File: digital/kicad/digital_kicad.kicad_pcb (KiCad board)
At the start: 2 copper layers, 14 parts, among them Q1 2N3904, Q2 2N3904, Q4 2N3904, SW1 SW_SPST

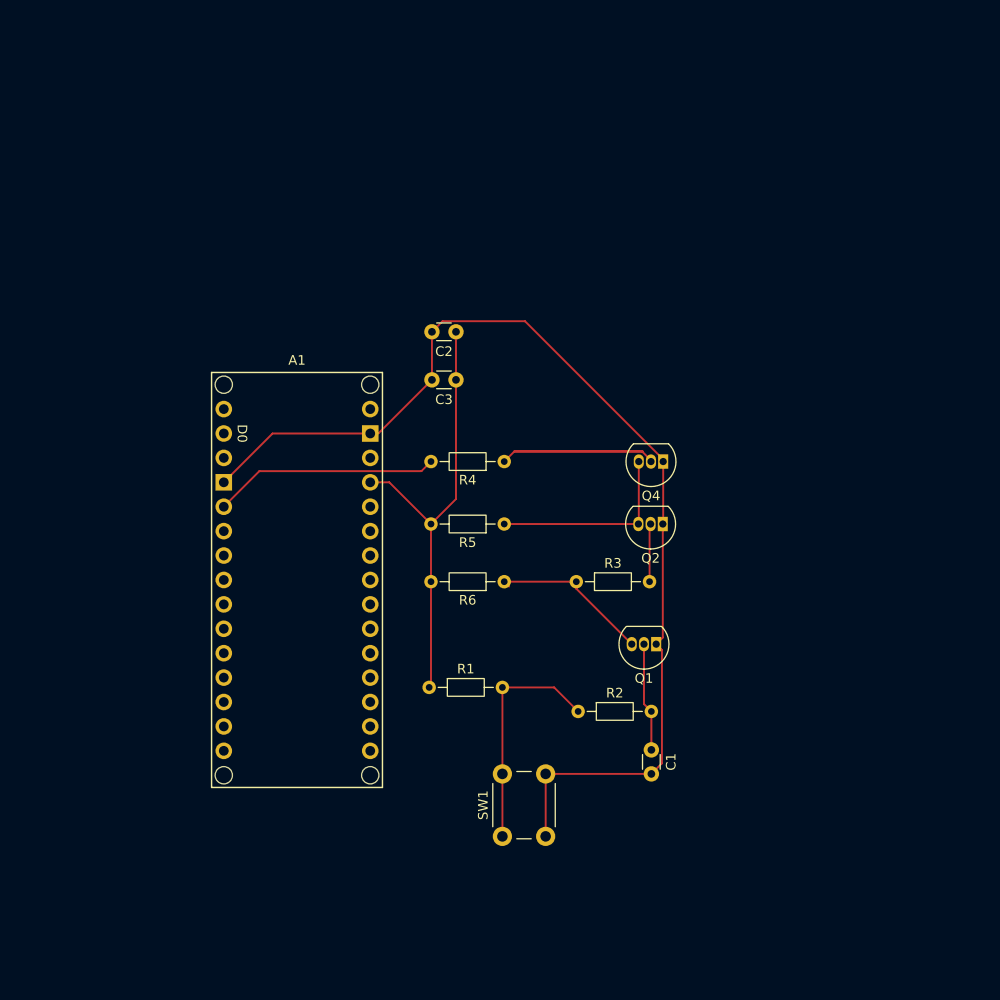
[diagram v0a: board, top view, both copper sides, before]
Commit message: kicad + pcb scheme review
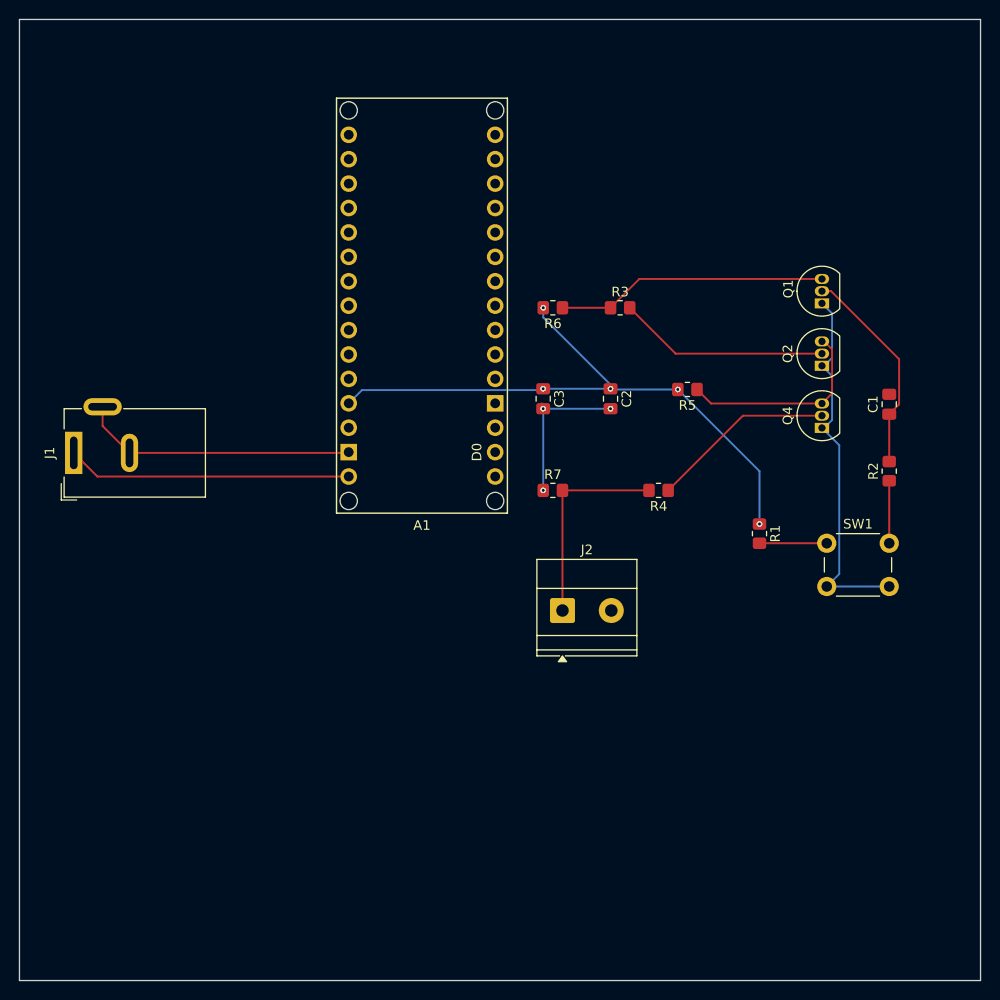
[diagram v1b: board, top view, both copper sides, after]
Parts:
- added J1: Barrel_Jack_Switch, Connector_BarrelJack:BarrelJack_Wuerth_6941xx301002, F.Cu at (105.7, 74.1)
- added J2: Screw_Terminal_01x02, TerminalBlock_Phoenix:TerminalBlock_Phoenix_MKDS-1,5-2-5.08_1x02_P5.08mm_Horizontal, F.Cu at (156.5, 90.5)
- added R7: 33k, Resistor_SMD:R_0805_2012Metric_Pad1.20x1.40mm_HandSolder, F.Cu at (155.5, 78.0)
- C1, C2, C3: footprint Capacitor_THT:C_Disc_D3.0mm_W1.6mm_P2.50mm -> Capacitor_SMD:C_0805_2012Metric_Pad1.18x1.45mm_HandSolder
- R1, R2, R3, R4, R5, R6: footprint Resistor_THT:R_Axial_DIN0204_L3.6mm_D1.6mm_P7.62mm_Horizontal -> Resistor_SMD:R_0805_2012Metric_Pad1.20x1.40mm_HandSolder
- moved A1 72.9 mm to (141.9, 37.2), turned to 180 degrees
- moved SW1 45.5 mm to (184.0, 83.5), turned to 0 degrees
- moved C1 43.7 mm to (190.5, 69.0), turned to 90 degrees
- moved R2 40.9 mm to (190.5, 76.0), turned to 90 degrees
- moved Q1 39.4 mm to (183.5, 58.5), turned to 90 degrees
- moved R1 37.9 mm to (177.0, 82.5), turned to -90 degrees
- moved R6 28.9 mm to (155.5, 59.0)
- moved R3 28.9 mm to (162.5, 59.0)
- moved R5 23.6 mm to (169.5, 67.5)
- moved Q2 23.3 mm to (183.5, 65.0), turned to 90 degrees
- moved C2 17.5 mm to (161.5, 68.5), turned to -90 degrees
- moved Q4 16.9 mm to (183.5, 71.5), turned to 90 degrees
- moved R4 16.3 mm to (166.5, 78.0)
- moved C3 9.28 mm to (154.5, 68.5), turned to -90 degrees
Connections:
- A1 pad D2: Net-(A1-D2_INT0) -> unconnected-(A1-D2_INT0-PadD2)
- A1 pad VIN: unconnected-(A1-PadVIN) -> /VDC
- R4 pad 2: Net-(A1-D2_INT0) -> Net-(J2-Pin_1)
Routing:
- net /VDC: track 0.00 -> 29.6 mm
- net GND: track 112.6 -> 83.8 mm, vias 0 -> 6
- net Net-(A1-D2_INT0): track 23.9 -> 0.00 mm
- net Net-(J2-Pin_1): track 0.00 -> 21.5 mm
- net +5V: track 46.7 -> 65.1 mm, vias 0 -> 6
- net Net-(Q2-B): track 6.05 -> 22.0 mm
- net inv. SW: track 17.1 -> 28.2 mm
- net SW: track 24.4 -> 13.5 mm
- net Net-(Q1-B): track 11.3 -> 22.0 mm
- net A: track 29.6 -> 19.2 mm
- net Net-(Q2-C): track 20.5 -> 21.1 mm
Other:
- board outline added: 100 x 100 mm
